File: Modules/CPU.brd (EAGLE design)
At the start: 132.1 x 55.9 mm, 92 parts, among them IC4 93LC66SM, IC5 MIC2026-1YM, IC8 AP2331W-7, J1 USB_A_SMT_FEMALE, J2 USB_A_SMT_FEMALE, J4 SD_CARD_SOCKET, Q1 DMG1012T-7, Q2 DMG1012T-7, Q3 DMG1012T-7, U5 LAN9512-JZX, U6 FSUSB42UMX, Y2 25MHz

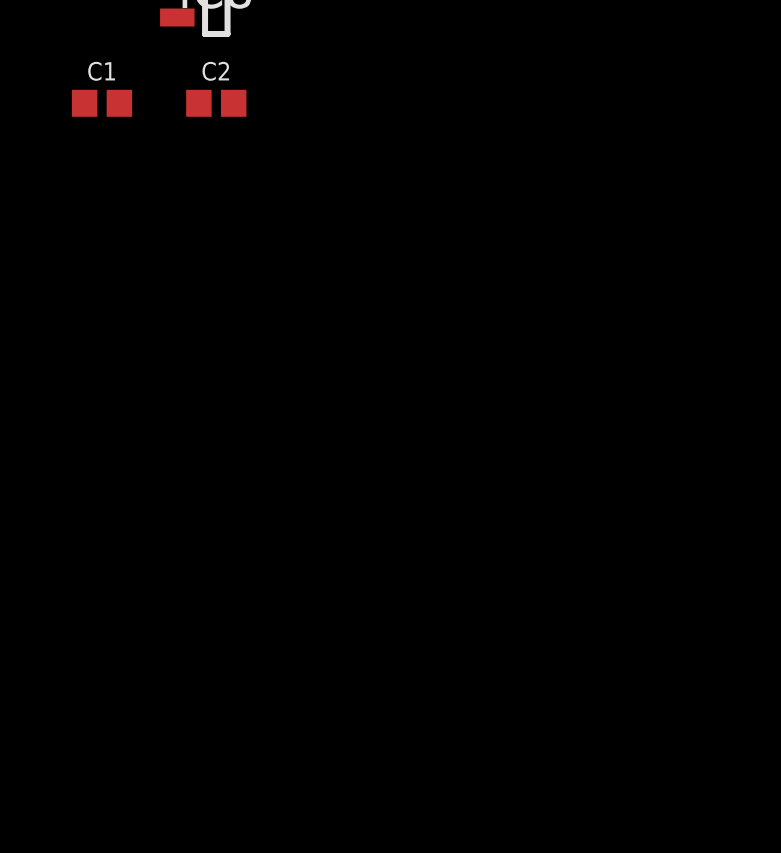
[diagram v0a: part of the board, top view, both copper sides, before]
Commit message: Merged HDMI
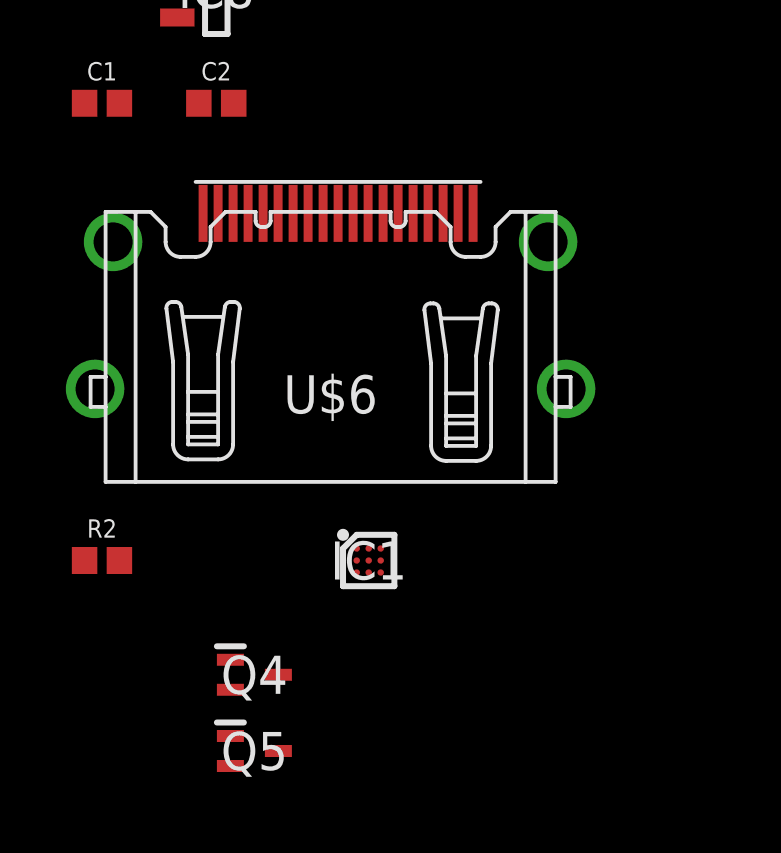
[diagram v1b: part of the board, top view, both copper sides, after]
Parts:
- added IC1: ESD5384NCTBG, SamacSys_Parts:BGA9C40P3X3_114X114X63
- added Q4, Q5: DMG1012T-7, SamacSys_Parts:SOT50P160X80-3N
- added R2: 100K, SparkFun-Resistors:0402
- added U$6: HDMI-A, connectors:HDMI_A
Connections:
- new net HDMI_CEC: CPU1.171, Q4.2
- new net HDMI_CK_N: CPU1.111, U$6.P$12
- new net HDMI_CK_P: CPU1.113, U$6.P$10
- new net HDMI_D0_N: CPU1.117, U$6.P$9
- new net HDMI_D0_P: CPU1.119, U$6.P$7
- new net HDMI_D1_N: CPU1.123, U$6.P$6
- new net HDMI_D1_P: CPU1.125, U$6.P$4
- new net HDMI_D2_N: CPU1.129, U$6.P$3
- new net HDMI_D2_P: CPU1.131, U$6.P$1
- new net HDMI_HPD_N_1V8: CPU1.88, Q5.3, R2.2
- new net HDMI_SCL: CPU1.175, IC1.B3, U$6.P$16
- new net HDMI_SDA: CPU1.173, IC1.A3, U$6.P$15
- new net N$6: IC1.C3, Q5.1, U$6.P$19
- new net N$9: IC1.A2, Q4.3, U$6.P$13
- net 1.8V: now also R2.1
- net GND: now also IC1.B2, IC1.C2, Q5.2, U$6.P$11, U$6.P$17, U$6.P$2, U$6.P$5, U$6.P$8
- net H5V: now also IC1.A1, IC1.C1, Q4.1, U$6.P$18

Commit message: Work
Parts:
- added SJ10: (no value), jumper:SJ
- moved Q4 172.3 mm to (67.3, 44.5)
- moved R2 165.6 mm to (57.1, 43.2)
- moved Q5 165.4 mm to (61.0, 39.4)
- moved IC1 162.6 mm to (62.2, 44.5)
- moved U$6 160.9 mm to (59.7, 50.8), turned to 180 degrees
- moved C2 154.6 mm to (54.6, 44.5)
- moved C1 151.1 mm to (49.5, 36.8)
- moved IC8 147.8 mm to (49.5, 41.9)
- moved C13 129.8 mm to (38.1, 85.1)
- moved C18 115.6 mm to (14.0, 29.2)
- moved FB1 109.6 mm to (14.0, 34.3)
- moved C12 105.4 mm to (-2.54, 30.5)
- moved C11 87.3 mm to (12.7, 64.8)
- moved C16 87.3 mm to (8.89, 64.8)
- moved C17 87.3 mm to (5.08, 64.8)
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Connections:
- net HDMI_CEC: now also SJ10.2
